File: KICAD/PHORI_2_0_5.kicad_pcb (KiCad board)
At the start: 2 copper layers, 125 x 80.9 mm, 113 parts, among them J1 Conn_01x06_Female, J2 Conn_01x02, J2 Conn_01x04_Female, J4 Conn_01x01, J4 Conn_01x04_Male, J5 Rumble, J6 PinSocket_1x04_P2.00mm_Vertic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, J9 USB_B_Micro, Q1 Q_NMOS_GSD, Q2 Q_PMOS_GDS, Q3 Q_NMOS_GSD, SW1 A, SW10 Dup, SW11 Dright, SW2 B, SW4 Y, SW5 Start, SW6 L, SW7 R, SW8 Z, U1 MCP3002, U10 DRV5055Z3QDBZT, U11 DRV5055Z3QDBZT, U12 USBLC6-2P6, U13 USBLC6-2P6, U2 Stickbox_Assembly_Main, U5 Stickbox_Assembly, U6 AMS1117-3.3, U7 W25Q128JVS, U8 RP2040, Y1 Crystal_GND24

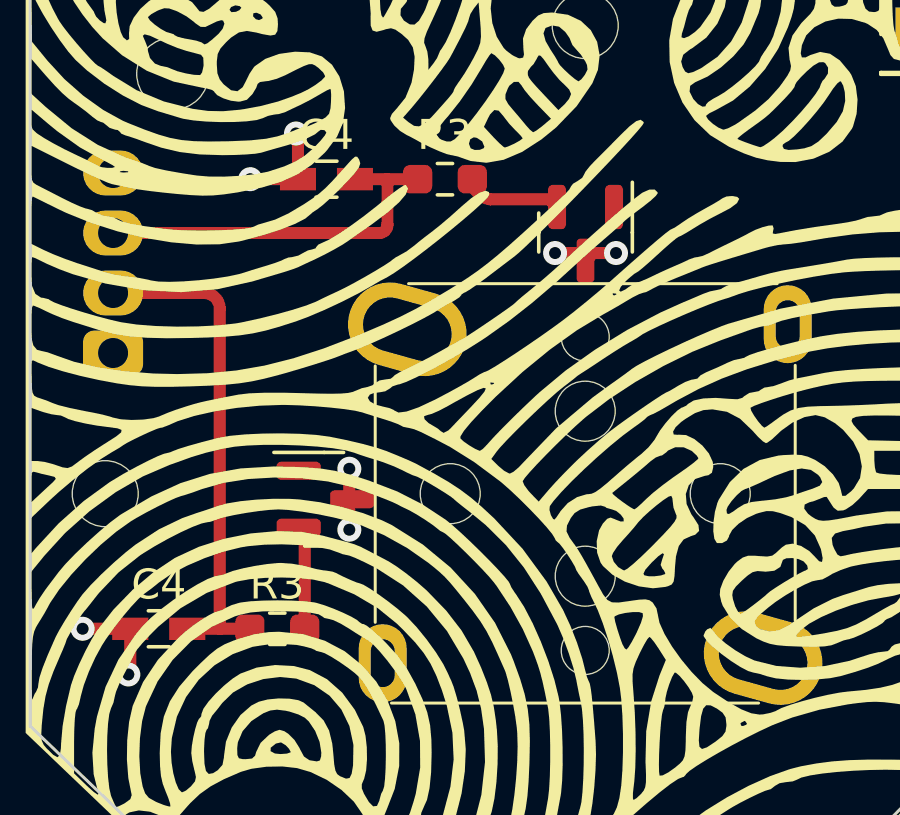
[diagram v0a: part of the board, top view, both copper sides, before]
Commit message: Updated JLC files
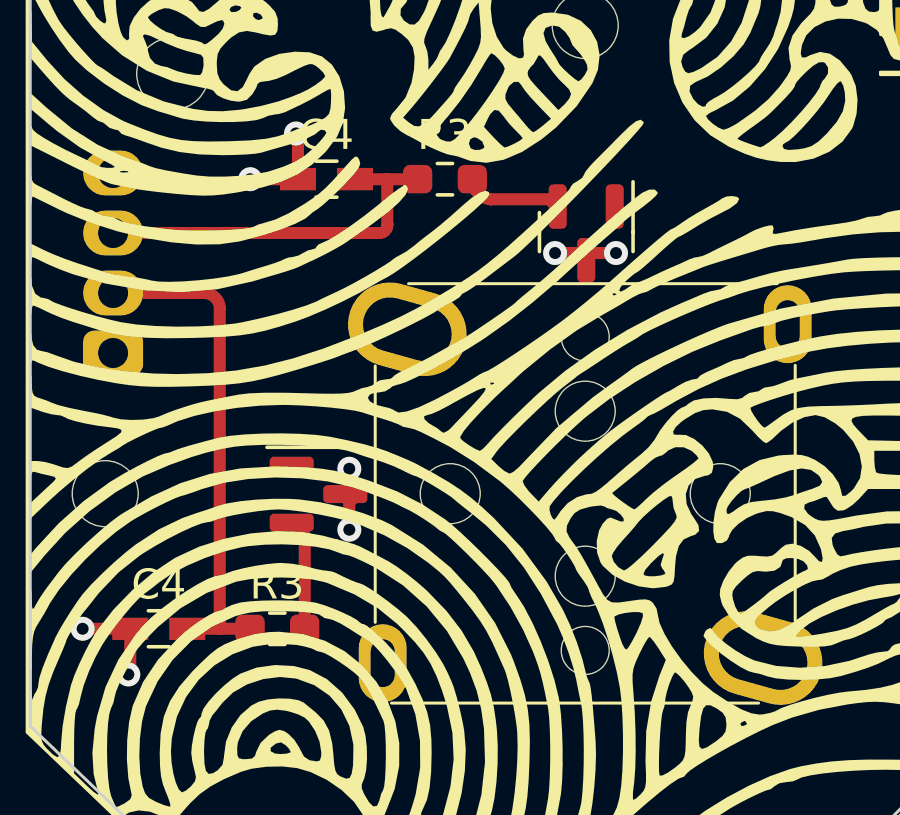
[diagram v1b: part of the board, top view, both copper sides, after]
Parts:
- moved U11 0.29 mm to (188.5, 114.9)
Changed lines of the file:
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@@
   )
   (footprint "PhobGCC_2_0_0_footprints:SOT-23" (layer "F.Cu")
-    (at 188.696875 115.095438)
+    (at 188.466397 114.924301)
     (descr "SOT, 3 Pin (https://www.jedec.org/system/files/docs/to-236h.pdf variant AB), generated with kicad-footprint-generator ipc_gullwing_generator.py")
     (tags "SOT TO_SOT_SMD")
@@
   )
   (footprint "PhobGCC_2_0_0_footprints:SOT-23" (layer "F.Cu")
-    (at 197.410875 106.204438 -90)
+    (at 197.434127 106.189462 -90)
     (descr "SOT, 3 Pin (https://www.jedec.org/system/files/docs/to-236h.pdf variant AB), generated with kicad-footprint-generator ipc_gullwing_generator.py")
     (tags "SOT TO_SOT_SMD")
@@
   (segment (start 146.206875 60.741938) (end 146.206875 58.072636) (width 0.15) (layer "F.Cu") (net 0))
   (segment (start 129.471875 66.614438) (end 127.081875 66.614438) (width 0.3) (layer "F.Cu") (net 0))
-  (segment (start 188.049375 119.413438) (end 188.049375 116.247938) (width 0.4) (layer "F.Cu") (net 0))
   (segment (start 150.731875 70.391438) (end 150.731875 70.021048) (width 0.15) (layer "F.Cu") (net 0))
   (segment (start 147.006875 60.741938) (end 147.006875 58.003583) (width 0.15) (layer "F.Cu") (net 0))
@@
   (segment (start 150.935038 61.647675) (end 151.894075 60.688638) (width 0.15) (layer "F.Cu") (net 0))
   (segment (start 152.198875 71.661438) (end 152.356559 71.503754) (width 0.15) (layer "F.Cu") (net 0))
+  (segment (start 188.049375 119.413438) (end 188.049375 116.307279) (width 0.4) (layer "F.Cu") (net 0))
   (segment (start 163.411955 59.976822) (end 163.545257 59.979438) (width 0.3) (layer "F.Cu") (net 0))
   (segment (start 157.567875 69.340438) (end 160.361875 72.134438) (width 0.15) (layer "F.Cu") (net 0))
@@
   (segment (start 151.295934 70.725221) (end 151.025296 70.995859) (width 0.15) (layer "F.Cu") (net 0))
   (segment (start 135.406875 54.417438) (end 135.434875 54.389438) (width 0.3) (layer "F.Cu") (net 0))
-  (segment (start 188.049375 116.247938) (end 187.846875 116.045438) (width 0.4) (layer "F.Cu") (net 0))
   (segment (start 99.029375 92.599438) (end 98.959375 92.529438) (width 0.25) (layer "F.Cu") (net 0))
   (segment (start 154.230875 66.835438) (end 154.230875 68.122354) (width 0.15) (layer "F.Cu") (net 0))
@@
   (segment (start 101.209375 99.366938) (end 101.216875 99.359438) (width 0.2) (layer "F.Cu") (net 0))
   (segment (start 128.706875 67.779438) (end 128.601875 67.884438) (width 0.3) (layer "F.Cu") (net 0))
+  (segment (start 188.049375 116.307279) (end 187.616397 115.874301) (width 0.4) (layer "F.Cu") (net 0))
   (segment (start 154.183435 69.327998) (end 156.684289 69.327998) (width 0.15) (layer "F.Cu") (net 0))
   (segment (start 190.806875 104.427438) (end 191.812375 104.427438) (width 0.4) (layer "F.Cu") (net 0))
